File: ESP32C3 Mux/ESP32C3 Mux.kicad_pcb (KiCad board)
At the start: 2 copper layers, 13 parts, among them J1 6130XX243121_613020243121, J2 Conn_01x02_Socket, U1 ESP32C3, U2 TCA9548APWR, U8 STLQ015M33R

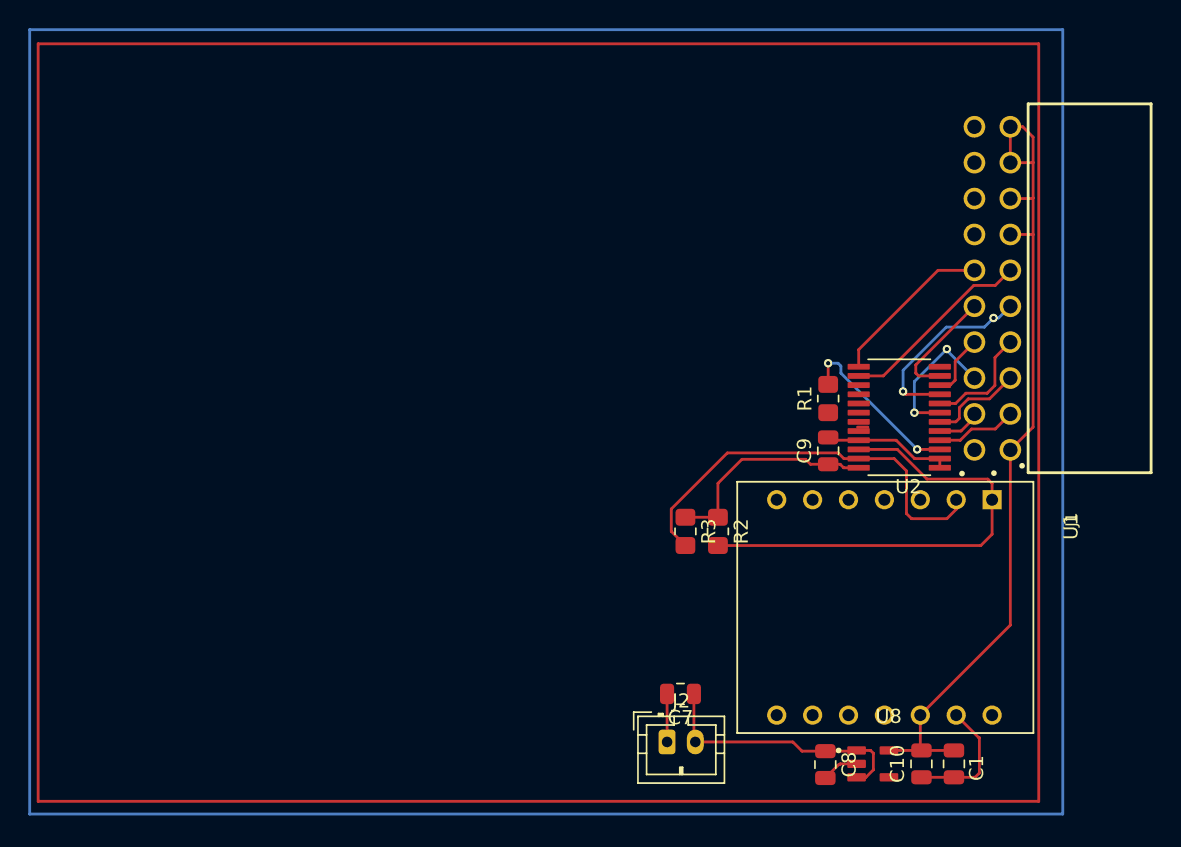
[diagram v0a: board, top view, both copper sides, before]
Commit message: finished layout
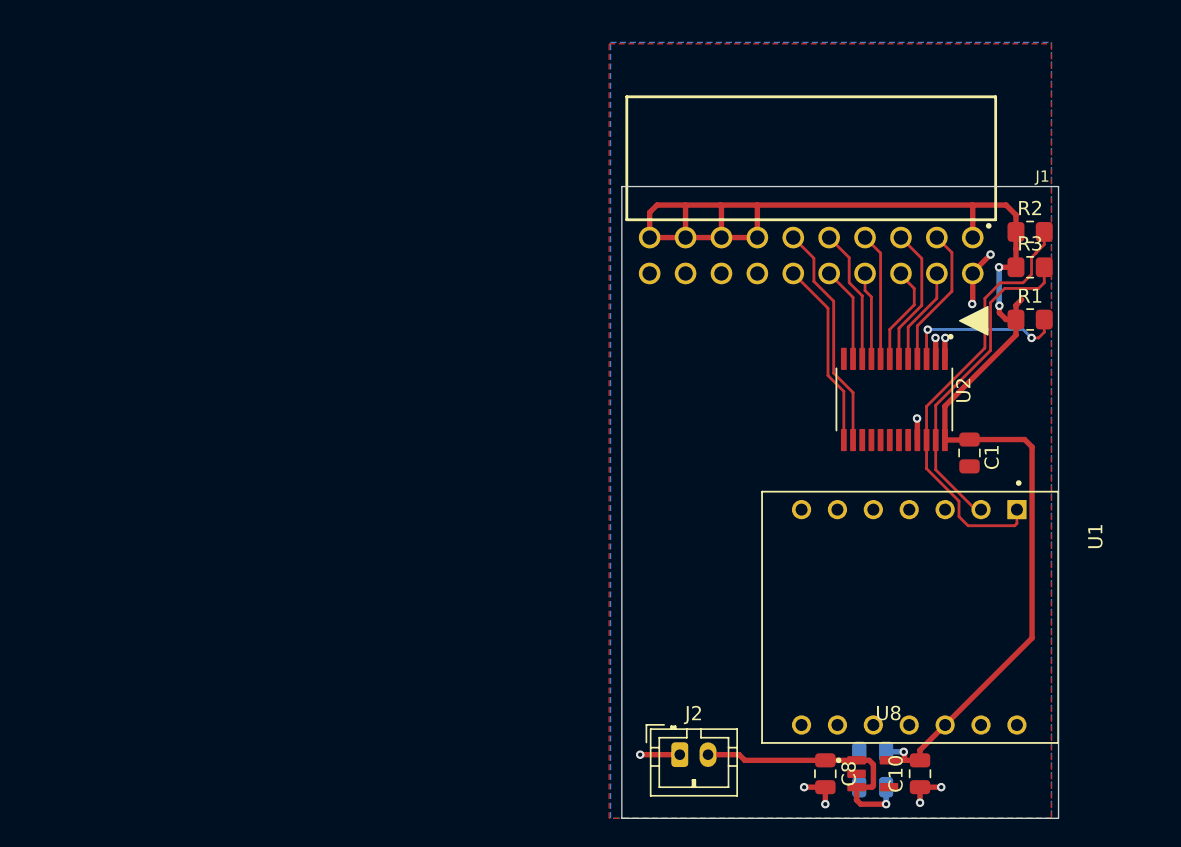
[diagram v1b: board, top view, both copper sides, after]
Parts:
- C7, C9: moved to B.Cu
- moved R3 30.7 mm to (174.6, 89.8), turned to 0 degrees
- moved R2 30.6 mm to (174.6, 87.3), turned to 0 degrees
- moved C1 22.0 mm to (170.3, 103.0)
- moved J1 21.7 mm to (159.1, 82.1), turned to 180 degrees
- moved C9 21.5 mm to (163.5, 124.1), turned to 180 degrees
- moved R1 15.3 mm to (174.6, 93.5), turned to 0 degrees
- moved C7 15.1 mm to (163.4, 126.6)
- moved U1 1.89 mm to (166.1, 114.6)
- moved U2 1.31 mm to (165.0, 99.2), turned to -90 degrees
- moved J2 1.27 mm to (149.8, 124.3)
- moved C10 0.71 mm to (166.8, 125.7)
- moved U8 0.70 mm to (163.5, 125.7)
- moved C8 0.65 mm to (160.1, 125.7)
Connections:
- J1 pad 8: /SDA3 -> /SCL2
- J1 pad 9: /SCL2 -> /SDA3
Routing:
- net +3V3: track 76.3 -> 102.7 mm, vias 0 -> 3
- net GND: track 24.2 -> 16.7 mm, vias 0 -> 10
- net /SCL2: track 13.6 -> 6.23 mm, vias 2 -> 0
- net /SDA: track 29.5 -> 23.3 mm
- net /SDA3: track 4.49 -> 9.55 mm
- net /SDA0: track 5.76 -> 10.0 mm
- net /SCL0: track 3.10 -> 6.89 mm
- net /SDA1: track 6.71 -> 9.86 mm
- net /SCL1: track 10.1 -> 7.15 mm, vias 2 -> 0
- net /SCL: track 33.8 -> 30.9 mm
- net /SCL4: track 13.8 -> 16.1 mm
- net /SDA4: track 11.7 -> 13.3 mm
- net /SCL3: track 8.23 -> 6.75 mm
- net /SDA2: track 7.94 -> 9.04 mm
- net unconnected-(U2-SC7-Pad20): track 0.74 -> 0.00 mm
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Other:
- board outline added: 30.9 x 44.7 mm
